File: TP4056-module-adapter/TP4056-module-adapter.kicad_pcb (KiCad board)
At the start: 2 copper layers, 25.9 x 8.5 mm, 11 parts, among them J1 Conn_01x01, J2 Conn_01x01, J3 Conn_01x01, J4 Conn_01x01, J5 Conn_01x01, Q1 SI2301, Q2 SI2301

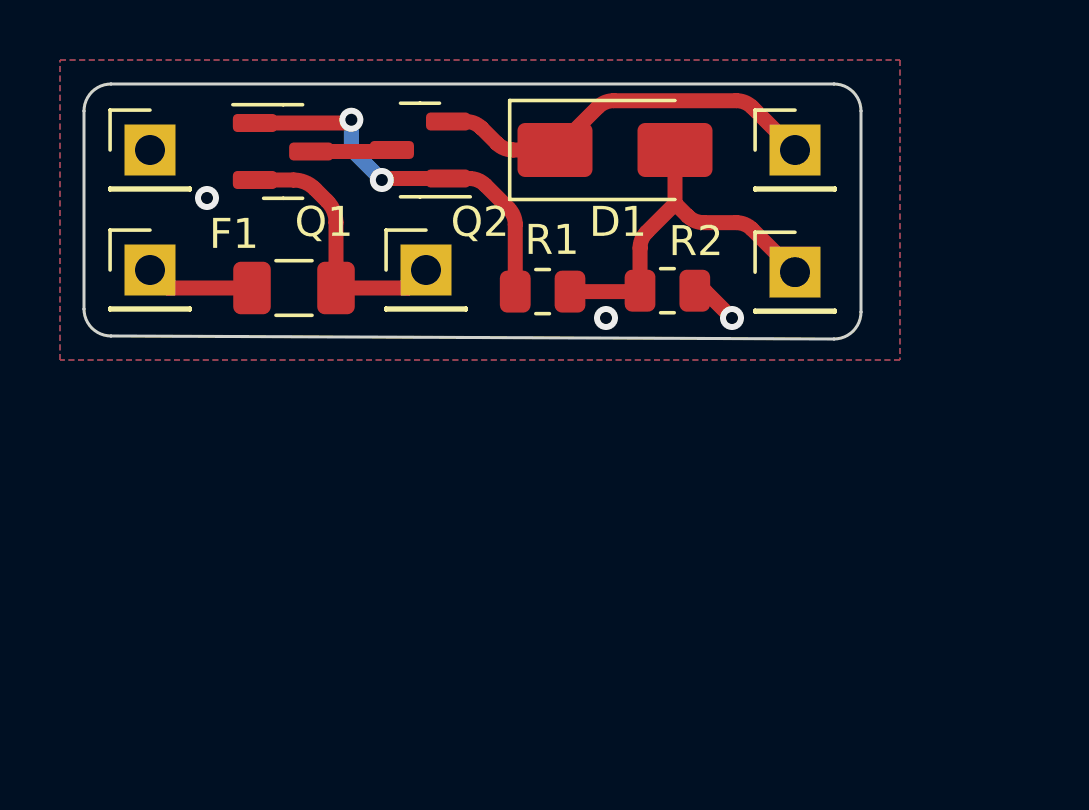
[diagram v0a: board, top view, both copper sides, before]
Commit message: v1.2 - ready for ordering
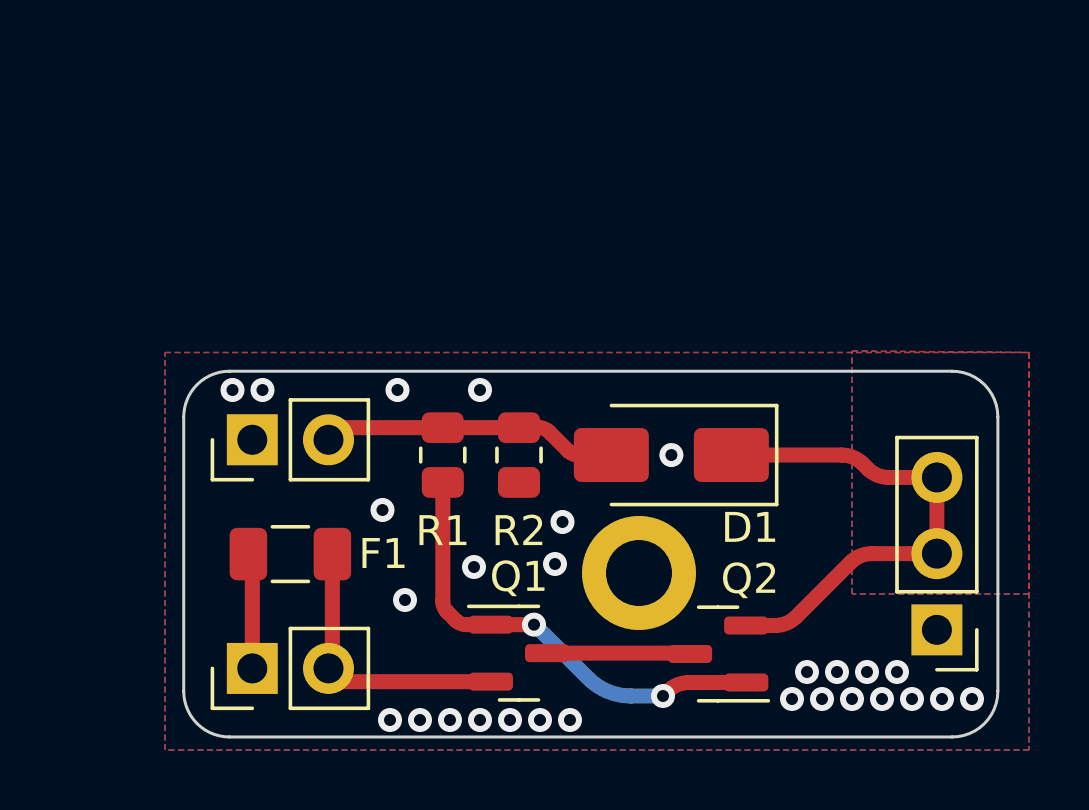
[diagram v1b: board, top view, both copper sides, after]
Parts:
- removed J4, J5: Conn_01x01, Connector_PinHeader_2.54mm:PinHeader_1x01_P2.54mm_Vertical
- added H1: MountingHole, MountingHole:MountingHole_2.2mm_M2_DIN965_Pad, F.Cu at (118.3, 78.1)
- J1, J2: value Conn_01x01 -> Conn_01x02; footprint Connector_PinHeader_2.54mm:PinHeader_1x01_P2.54mm_Vertical -> Connector_PinHeader_2.54mm:PinHeader_1x02_P2.54mm_Vertical
- J3: value Conn_01x01 -> Conn_01x03; footprint Connector_PinHeader_2.54mm:PinHeader_1x01_P2.54mm_Vertical -> Connector_PinHeader_2.54mm:PinHeader_1x03_P2.54mm_Vertical
- moved J3 20.8 mm to (128.2, 80.0), turned to 180 degrees
- moved Q2 19.5 mm to (120.9, 80.8)
- moved J1 18.9 mm to (105.4, 73.7), turned to 90 degrees
- moved Q1 18.5 mm to (114.3, 80.8)
- moved J2 17.6 mm to (105.4, 81.3), turned to 90 degrees
- moved D1 10.3 mm to (119.4, 74.2), turned to 180 degrees
- moved F1 8.87 mm to (106.7, 77.5)
- moved R2 7.38 mm to (114.3, 74.2), turned to -90 degrees
- moved R1 6.38 mm to (111.8, 74.2), turned to 90 degrees
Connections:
- J1 pad 1: VBUS -> GND
- J2 pad 1: GND -> +BATT
- J3 pad 1: LINE -> GND
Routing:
- net VCC: track 13.2 -> 16.9 mm
- net VBUS: track 12.4 -> 9.93 mm
- net Net-(Q1-G): track 13.1 -> 15.5 mm
- net Net-(Q1-D): track 2.71 -> 4.77 mm
- net GND: track 1.62 -> 0.00 mm, vias 3 -> 28
- net LINE: track 8.87 -> 9.46 mm
- added copper zone on B.Cu, net VCC
- added copper zone on F.Cu, net VCC
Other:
- board size 25.9 x 8.5 mm -> 27.1 x 12.2 mm
- board text added: "Potpurri TP4056 MA, v1.2"
- board text removed: "Potpurri TP4056 MA, v1.0"
